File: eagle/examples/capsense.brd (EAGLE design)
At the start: 16.5 x 25.1 mm, 3 parts

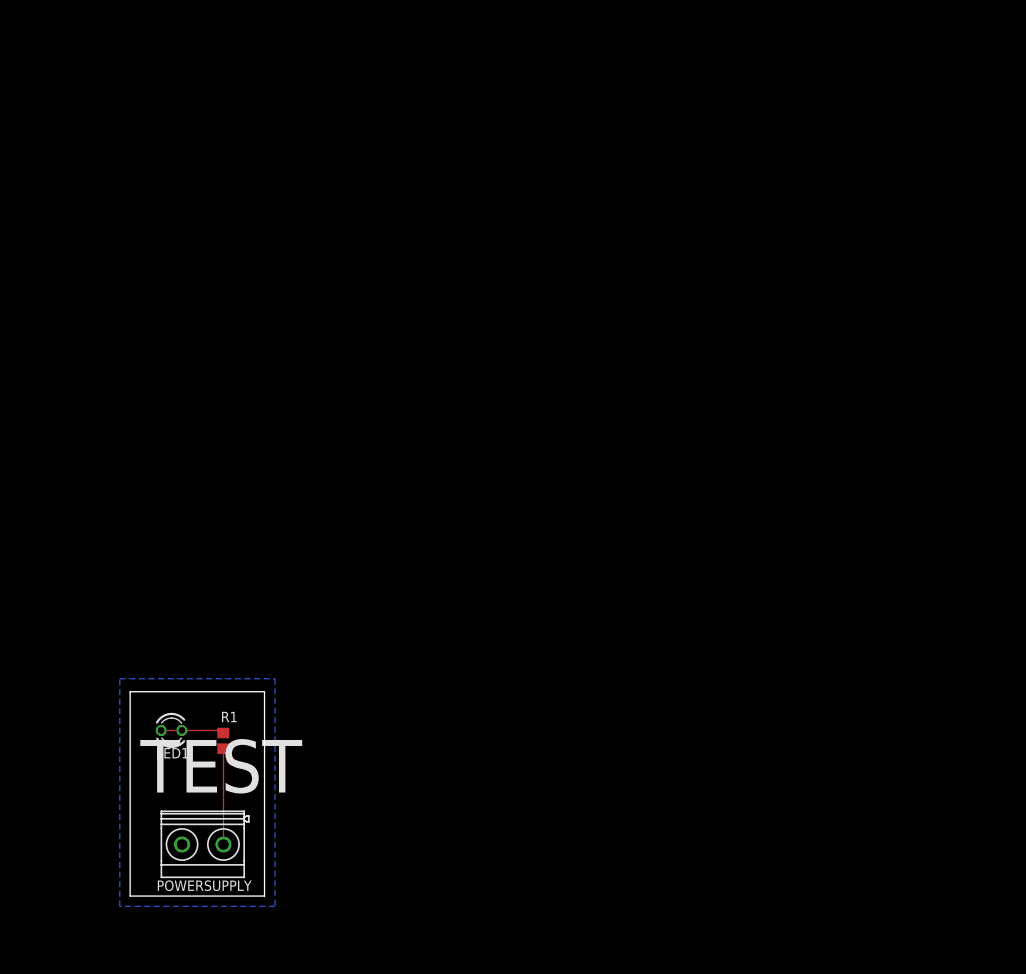
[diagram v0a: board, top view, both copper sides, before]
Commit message: examples
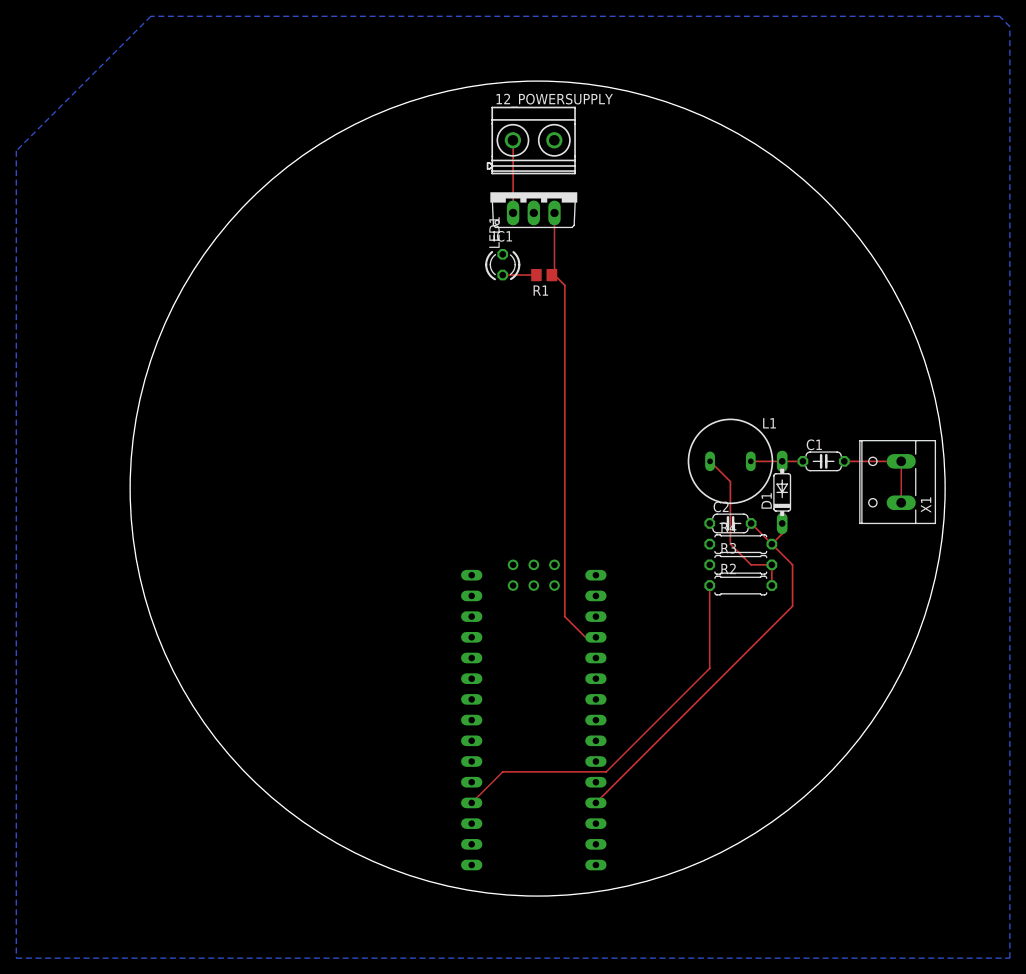
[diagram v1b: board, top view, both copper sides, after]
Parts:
- removed POWERSUPPLY: MKDSN1,5/2-5,08, con-phoenix-508:MKDSN1,5/2-5,08
- added 12_POWERSUPPLY: MKDSN1,5/2-5,08, con-phoenix-508:MKDSN1,5/2-5,08
- added C1: 10nF, rcl:C050-024X044
- added C2: 100nF, rcl:C050-024X044
- added D1: 1N4148DO35-7, diode:DO35-7
- added IC1: 7805TV, linear:TO220V
- added L1: 10mH, inductor-neosid:BS11
- added R2: 10K, rcl:0207/7
- added R3: 3k3, rcl:0207/7
- added R4: 1M, rcl:0207/7
- added U$1: NANO, Arduino-clone:NANO
- added X1: (no value), con-wago-508:W237-132
- moved LED1 70.1 mm to (45.7, 77.5), turned to 90 degrees
- moved R1 69.4 mm to (50.8, 76.2), turned to 180 degrees
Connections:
- new net +12V: 12_POWERSUPPLY.1, IC1.1
- new net N$1: R2.1, U$1.D9
- new net N$2: L1.1, R2.2, R3.2
- new net N$3: C1.1, D1.A, L1.2
- new net N$4: C1.2, X1.1, X1.2
- new net N$5: C2.2, D1.C, R4.2, U$1.A0
- net +5V: now also IC1.3, U$1.5V; no longer POWERSUPPLY.1
- net GND: now also 12_POWERSUPPLY.2, C2.1, IC1.2, R3.1, R4.1, U$1.GND; no longer POWERSUPPLY.2
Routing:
- net N$5: track 0.00 -> 49.5 mm
- net N$1: track 0.00 -> 46.2 mm
- net +5V: track 11.8 -> 55.4 mm
- net N$2: track 0.00 -> 19.9 mm
- net N$4: track 0.00 -> 12.1 mm
- net +12V: track 0.00 -> 8.92 mm
- net N$3: track 0.00 -> 6.39 mm
- net CONNECT: track 7.75 -> 4.13 mm
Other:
- board size 16.5 x 25.1 mm -> 100 x 100 mm
- board text removed: "TEST"
